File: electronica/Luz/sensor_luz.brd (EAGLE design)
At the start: 40 x 20 mm, 13 parts

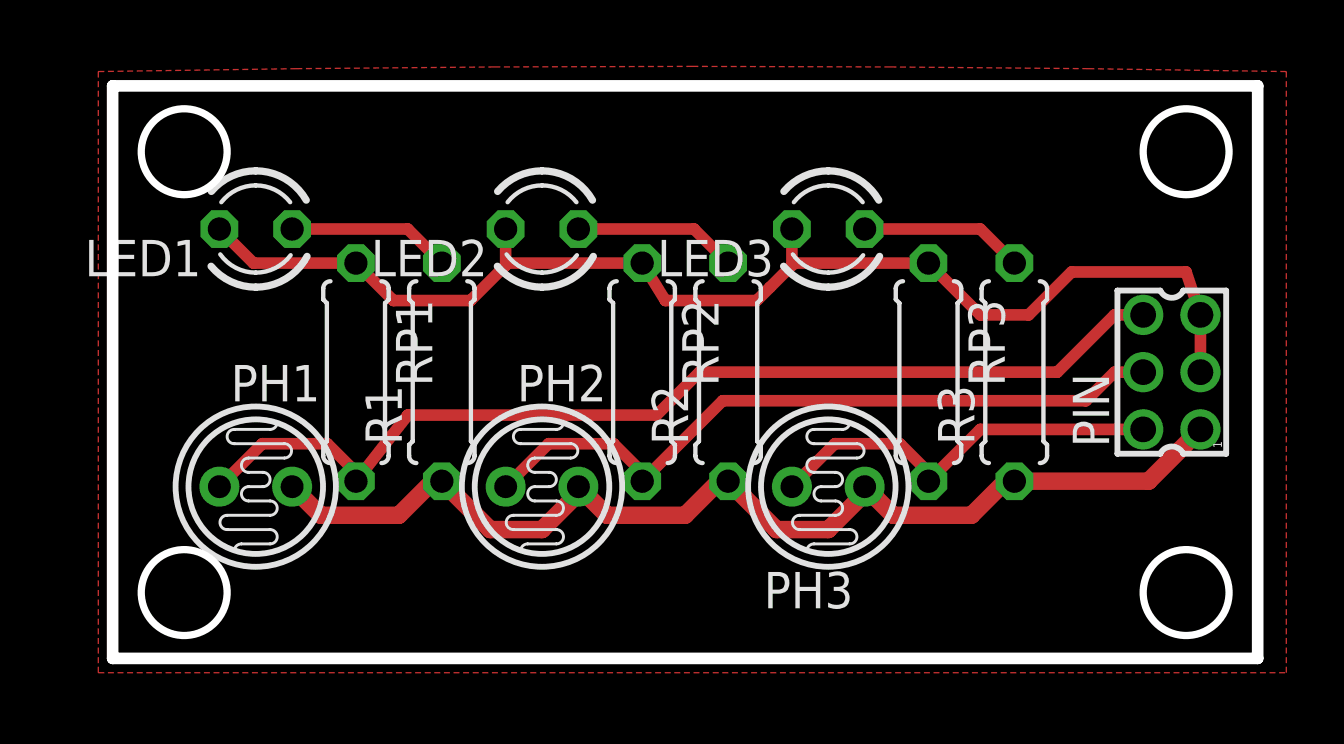
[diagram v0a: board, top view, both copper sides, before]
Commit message: electronica sensor luz
ajustes finales
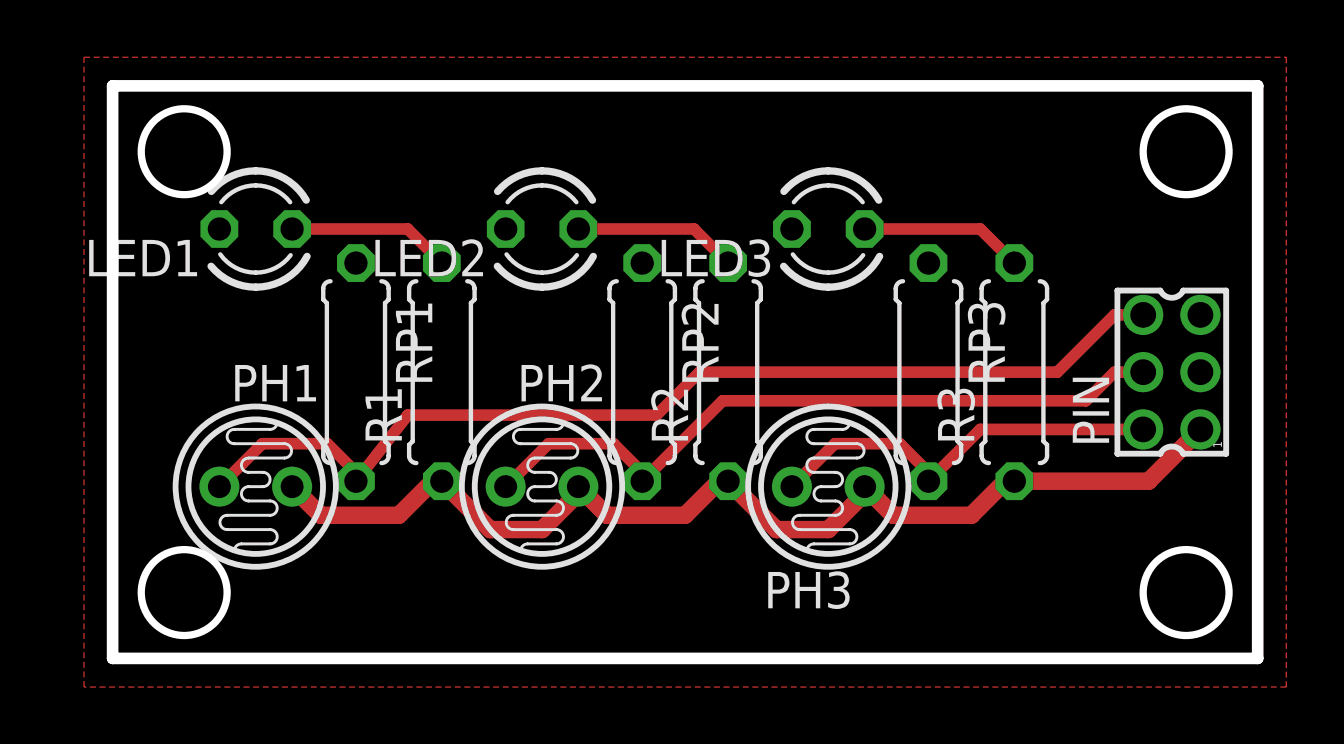
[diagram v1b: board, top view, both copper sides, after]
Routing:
- net GND: track 44.1 -> 0.00 mm
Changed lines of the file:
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@@
 <setting verticaltext="up"/>
 </settings>
-<grid distance="0.003125" unitdist="mic" unit="mm" style="lines" multiple="1" display="yes" altdistance="0.003125" altunitdist="mic" altunit="mm"/>
+<grid distance="1" unitdist="mm" unit="mm" style="lines" multiple="1" display="yes" altdistance="1" altunitdist="mm" altunit="mm"/>
 <layers>
 <layer number="1" name="Top" color="4" fill="1" visible="yes" active="yes"/>
@@
 <layer number="14" name="Route14" color="1" fill="6" visible="no" active="no"/>
 <layer number="15" name="Route15" color="4" fill="6" visible="no" active="no"/>
-<layer number="16" name="Bottom" color="1" fill="1" visible="no" active="yes"/>
+<layer number="16" name="Bottom" color="1" fill="1" visible="yes" active="yes"/>
 <layer number="17" name="Pads" color="2" fill="1" visible="yes" active="yes"/>
 <layer number="18" name="Vias" color="2" fill="1" visible="yes" active="yes"/>
@@
 <contactref element="LED3" pad="K"/>
 <contactref element="LED2" pad="K"/>
-<wire x1="8.5" y1="13.81" x2="4.92" y2="13.81" width="0.4064" layer="1"/>
-<wire x1="4.92" y1="13.81" x2="3.73" y2="15" width="0.4064" layer="1"/>
 <contactref element="PIN" pad="5"/>
-<wire x1="38" y1="12" x2="37.5" y2="13.5" width="0.4064" layer="1"/>
-<wire x1="37.5" y1="13.5" x2="33.5" y2="13.5" width="0.4064" layer="1"/>
-<wire x1="33.5" y1="13.5" x2="32" y2="12" width="0.4064" layer="1"/>
-<wire x1="32" y1="12" x2="30.31" y2="12" width="0.4064" layer="1"/>
-<wire x1="30.31" y1="12" x2="28.5" y2="13.81" width="0.4064" layer="1"/>
-<wire x1="23.73" y1="15" x2="23.73" y2="13.73" width="0.4064" layer="1"/>
-<wire x1="23.73" y1="13.73" x2="22.960903125" y2="12.960903125" width="0.4064" layer="1"/>
-<wire x1="22.960903125" y1="12.960903125" x2="22.5" y2="12.5" width="0.4064" layer="1"/>
-<wire x1="22.5" y1="12.5" x2="19.31" y2="12.5" width="0.4064" layer="1"/>
-<wire x1="19.31" y1="12.5" x2="18.5" y2="13.81" width="0.4064" layer="1"/>
-<wire x1="13.73" y1="15" x2="13.73" y2="13.73" width="0.4064" layer="1"/>
-<wire x1="13.73" y1="13.73" x2="12.5" y2="12.5" width="0.4064" layer="1"/>
-<wire x1="12.5" y1="12.5" x2="9.81" y2="12.5" width="0.4064" layer="1"/>
-<wire x1="9.81" y1="12.5" x2="8.5" y2="13.81" width="0.4064" layer="1"/>
 <contactref element="PIN" pad="3"/>
-<wire x1="38" y1="10" x2="38" y2="12" width="0.4064" layer="1"/>
-<polygon width="1.016" layer="1" isolate="0.6096" orphans="yes">
-<vertex x="-0.5" y="20.5"/>
-<vertex x="-0.5" y="-0.5"/>
-<vertex x="41" y="-0.5"/>
-<vertex x="41" y="20.5" curve="2"/>
+<polygon width="1.016" layer="1" isolate="0.6096">
+<vertex x="-1" y="-1"/>
+<vertex x="-1" y="21"/>
+<vertex x="41" y="21"/>
+<vertex x="41" y="-1"/>
 </polygon>
-<wire x1="18.5" y1="13.81" x2="13.81" y2="13.81" width="0.4064" layer="1"/>
-<wire x1="13.81" y1="13.81" x2="13.73" y2="13.73" width="0.4064" layer="1"/>
-<wire x1="28.5" y1="13.81" x2="23.81" y2="13.81" width="0.4064" layer="1"/>
-<wire x1="23.81" y1="13.81" x2="23.73" y2="13.73" width="0.4064" layer="1"/>
 </signal>
 <signal name="N$2">
